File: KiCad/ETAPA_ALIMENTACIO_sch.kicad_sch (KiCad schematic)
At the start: 14 parts, among them U4 LM2596S-5, U6 LM1117DT-3.3

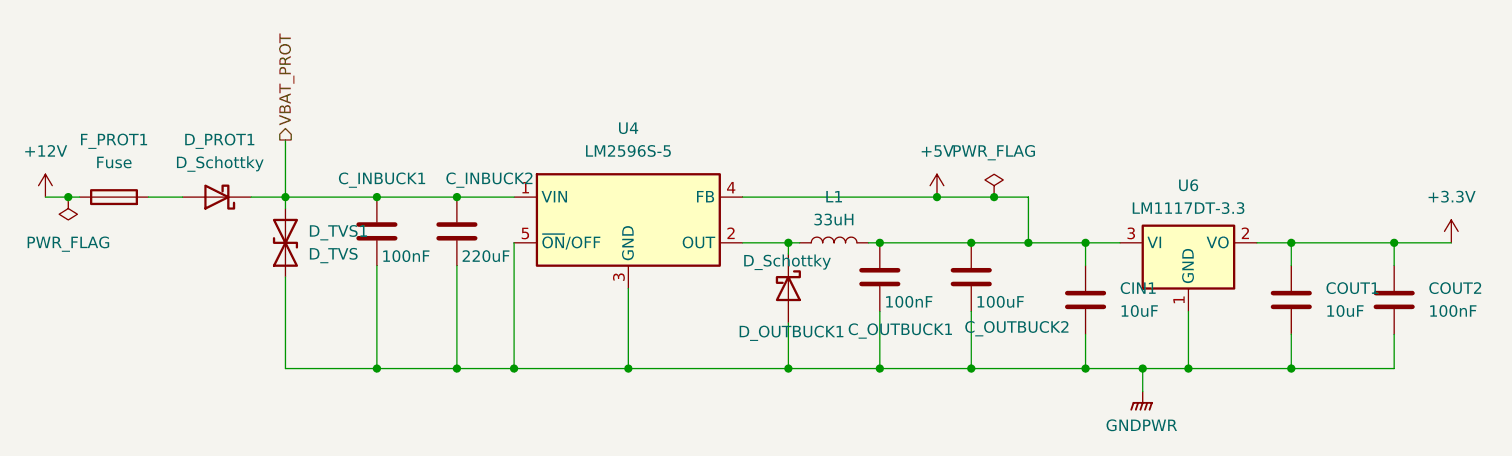
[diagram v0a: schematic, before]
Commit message: V1 Routing
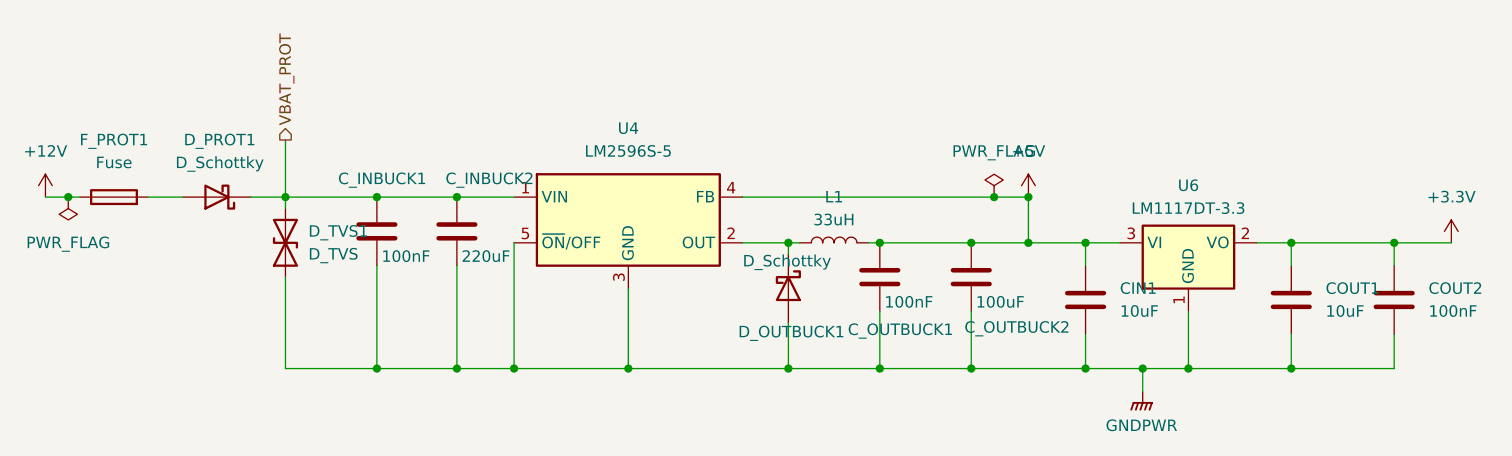
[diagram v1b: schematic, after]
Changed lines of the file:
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@@
+	)
+	(junction
+		(at 170.18 85.09)
+		(diameter 0)
+		(color 0 0 0 0)
 	)
 	(junction
@@
 	)
 	(junction
-		(at 160.02 85.09)
-		(diameter 0)
-		(color 0 0 0 0)
-	)
-	(junction
 		(at 199.39 104.14)
 		(diameter 0)
@@
 	(wire
 		(pts
-			(xy 160.02 85.09) (xy 166.37 85.09)
+			(xy 138.43 85.09) (xy 166.37 85.09)
 		)
 		(stroke
@@
 		(pts
 			(xy 182.88 104.14) (xy 187.96 104.14)
-		)
-		(stroke
-			(width 0)
-			(type default)
-		)
-	)
-	(wire
-		(pts
-			(xy 138.43 85.09) (xy 160.02 85.09)
 		)
 		(stroke
@@
 		(dnp no)
 		(fields_autoplaced yes)
-		(property "Reference" "#FLG07"
+		(property "Reference" "#FLG04"
 			(at 63.5 86.995 0)
 			(effects
@@
 			(project "PROJECTE_EINES"
 				(path "/347831db-5db9-4aff-ad32-e56fd770e219/b8d025f8-884e-44af-b29b-4fb2140b95b4"
-					(reference "#FLG07")
+					(reference "#FLG04")
 					(unit 1)
 				)
@@
 		(dnp no)
 		(fields_autoplaced yes)
-		(property "Reference" "#PWR050"
+		(property "Reference" "#PWR031"
 			(at 60.96 88.9 0)
 			(effects
@@
 			(project "PROJECTE_EINES"
 				(path "/347831db-5db9-4aff-ad32-e56fd770e219/b8d025f8-884e-44af-b29b-4fb2140b95b4"
-					(reference "#PWR050")
+					(reference "#PWR031")
 					(unit 1)
 				)
@@
 	)
 	(symbol
+		(lib_id "power:+5V")
+		(at 170.18 85.09 0)
+		(unit 1)
+		(exclude_from_sim no)
+		(in_bom yes)
+		(on_board yes)
+		(dnp no)
+		(fields_autoplaced yes)
+		(property "Reference" "#PWR049"
+			(at 170.18 88.9 0)
+			(effects
+				(font
+					(size 1.27 1.27)
+				)
+				(hide yes)
+			)
+		)
+		(property "Value" "+5V"
+			(at 170.18 80.01 0)
+			(effects
+				(font
+					(size 1.27 1.27)
+				)
+			)
+		)
+		(property "Footprint" ""
+			(at 170.18 85.09 0)
+			(effects
+				(font
+					(size 1.27 1.27)
+				)
+				(hide yes)
+			)
+		)
+		(property "Datasheet" ""
+			(at 170.18 85.09 0)
+			(effects
+				(font
+					(size 1.27 1.27)
+				)
+				(hide yes)
+			)
+		)
+		(property "Description" "Power symbol creates a global label with name \"+5V\""
+			(at 170.18 85.09 0)
+			(effects
+				(font
+					(size 1.27 1.27)
+				)
+				(hide yes)
+			)
+		)
+		(pin "1"
+		)
+		(instances
+			(project ""
+				(path "/347831db-5db9-4aff-ad32-e56fd770e219/b8d025f8-884e-44af-b29b-4fb2140b95b4"
+					(reference "#PWR049")
+					(unit 1)
+				)
+			)
+		)
+	)
+	(symbol
 		(lib_id "Device:C")
 		(at 97.79 88.9 0)
@@
 		(dnp no)
 		(fields_autoplaced yes)
-		(property "Reference" "#PWR040"
+		(property "Reference" "#PWR041"
 			(at 182.88 111.76 0)
 			(effects
@@
 			(project "PROJECTE_EINES"
 				(path "/347831db-5db9-4aff-ad32-e56fd770e219/b8d025f8-884e-44af-b29b-4fb2140b95b4"
-					(reference "#PWR040")
+					(reference "#PWR041")
 					(unit 1)
 				)
@@
 					(unit 1)
 				)
-			)
-		)
-	)
-	(symbol
-		(lib_id "power:+5V")
-		(at 160.02 85.09 0)
-		(unit 1)
-		(exclude_from_sim no)
-		(in_bom yes)
-		(on_board yes)
-		(dnp no)
-		(fields_autoplaced yes)
-		(property "Reference" "#PWR037"
-			(at 160.02 88.9 0)
-			(effects
-				(font
-					(size 1.27 1.27)
-				)
-				(hide yes)
-			)
-		)
-		(property "Value" "+5V"
-			(at 160.02 80.01 0)
-			(effects
-				(font
-					(size 1.27 1.27)
-				)
-			)
-		)
-		(property "Footprint" ""
-			(at 160.02 85.09 0)
-			(effects
-				(font
-					(size 1.27 1.27)
-				)
-				(hide yes)
-			)
-		)
-		(property "Datasheet" ""
-			(at 160.02 85.09 0)
-			(effects
-				(font
-					(size 1.27 1.27)
-				)
-				(hide yes)
-			)
-		)
-		(property "Description" "Power symbol creates a global label with name \"+5V\""
-			(at 160.02 85.09 0)
-			(effects
-				(font
-					(size 1.27 1.27)
-				)
-				(hide yes)
-			)
-		)
-		(pin "1"
-		)
-		(instances
-			(project "PROJECTE_EINES"
-				(path "/347831db-5db9-4aff-ad32-e56fd770e219/b8d025f8-884e-44af-b29b-4fb2140b95b4"
-					(reference "#PWR037")
-					(unit 1)
-				)
